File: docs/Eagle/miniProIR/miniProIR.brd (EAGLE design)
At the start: 41.7 x 24.6 mm, 13 parts, among them J4 Pixel, J7 Interface

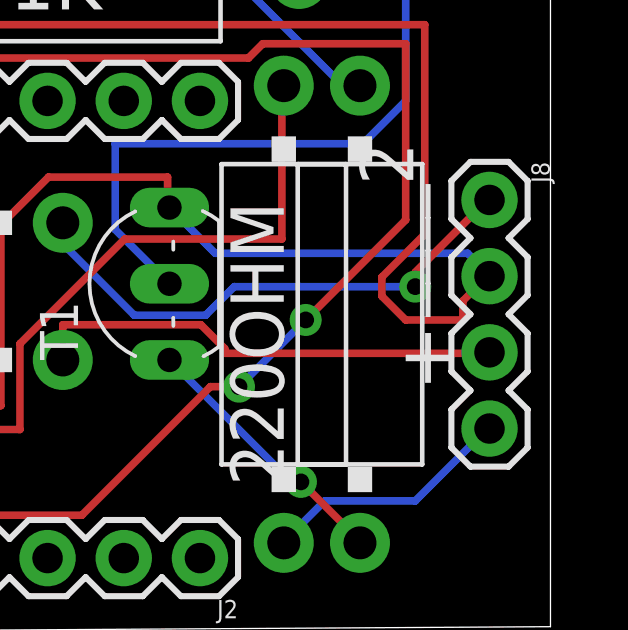
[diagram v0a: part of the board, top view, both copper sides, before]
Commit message: hyo
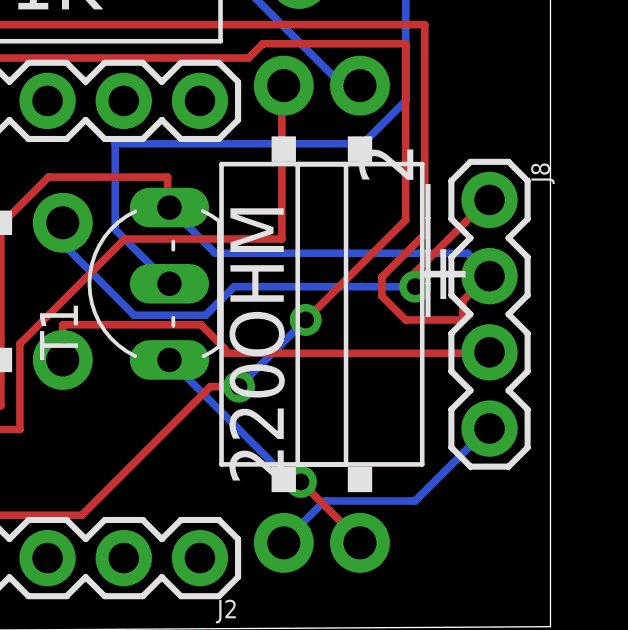
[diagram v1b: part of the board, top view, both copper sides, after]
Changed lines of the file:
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@@
 GND</text>
 <text x="23.622" y="20.828" size="1.9304" layer="121">1K</text>
-<text x="36.576" y="8.382" size="1.9304" layer="121">+</text>
+<text x="37.084" y="11.176" size="1.9304" layer="121">+</text>
 </plain>
 <attributes>
